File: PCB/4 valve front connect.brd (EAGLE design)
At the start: 82.6 x 57.5 mm, 17 parts, among them T1 2N2222, T2 2N2222, T3 2N2222

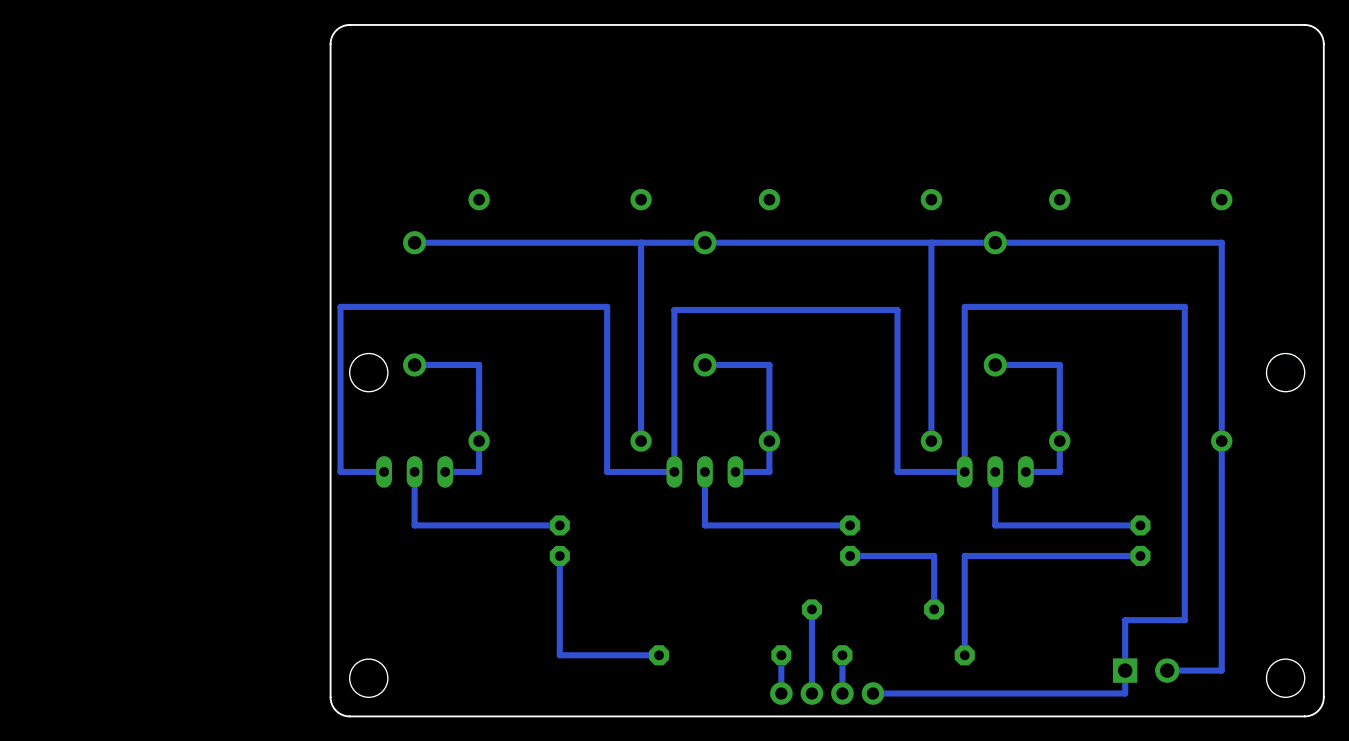
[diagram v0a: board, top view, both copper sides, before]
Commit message: 4 valve boards
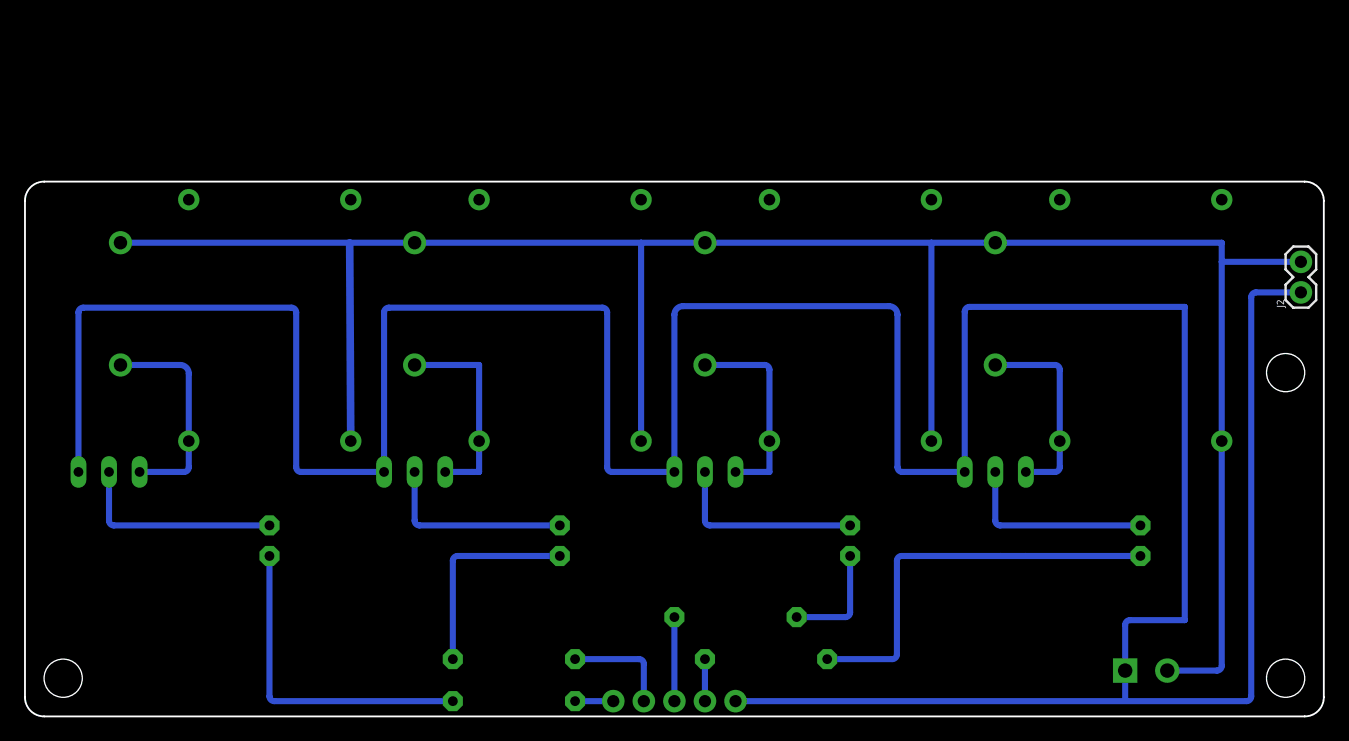
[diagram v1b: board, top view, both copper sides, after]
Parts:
- added D4: 1N4004, adafruit:DO41-10
- added J2: (no value), SparkFun-Connectors:1X02
- added LED4: (no value), adafruit:LED5MM
- added R4: (no value), adafruit:0207/10
- added T4: 2N2222, adafruit:TO92-EBC-OVAL
- added U$3: (no value), local eagle library:VALVTEST2
- SV1: device SparkFun-Connectors:1X04 -> SparkFun-Connectors:1X05
- moved R3 17.1 mm to (-29.2, 4.76)
- moved SV1 14.0 mm to (-21.0, 1.27)
- moved R2 11.4 mm to (-10.8, 8.26)
- moved R1 11.4 mm to (-8.26, 4.76)
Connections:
- removed net N$44: R2.1, SV1.2
- new net N$12: LED4.A, R4.2
- new net N$13: R4.1, SV1.1
- new net N$14: R2.1, SV1.3
- new net N$4: D4.A, T4.C, U$3.PAD11
- new net N$8: LED4.K, T4.B
- net 5V: now also D4.C, J2.2, U$3.PAD10
- net GND: now also J2.1, SV1.5, T4.E; no longer SV1.4
- net N$19: now also SV1.2; no longer SV1.1
- net N$30: now also SV1.4; no longer SV1.3
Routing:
- net GND: track 199.9 -> 303.2 mm
- net 5V: track 140.1 -> 187.4 mm, vias 0 -> 1
- net N$12: track 0.00 -> 27.1 mm
- net N$4: track 0.00 -> 18.0 mm
- net N$8: track 0.00 -> 17.5 mm
- net N$3: track 22.9 -> 34.1 mm
- net N$14: track 0.00 -> 6.99 mm
- net N$44: track 6.99 -> 0.00 mm
- net N$19: track 3.17 -> 8.98 mm
- net N$13: track 0.00 -> 3.18 mm
- net N$7: track 11.4 -> 9.29 mm
- net N$11: track 16.5 -> 17.2 mm
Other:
- board size 82.6 x 57.5 mm -> 107.9 x 44.5 mm
